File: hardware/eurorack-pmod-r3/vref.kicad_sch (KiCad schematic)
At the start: 6 parts, among them U8 LM4040DBZ-3 VREF, U9 TL072 OP AMP

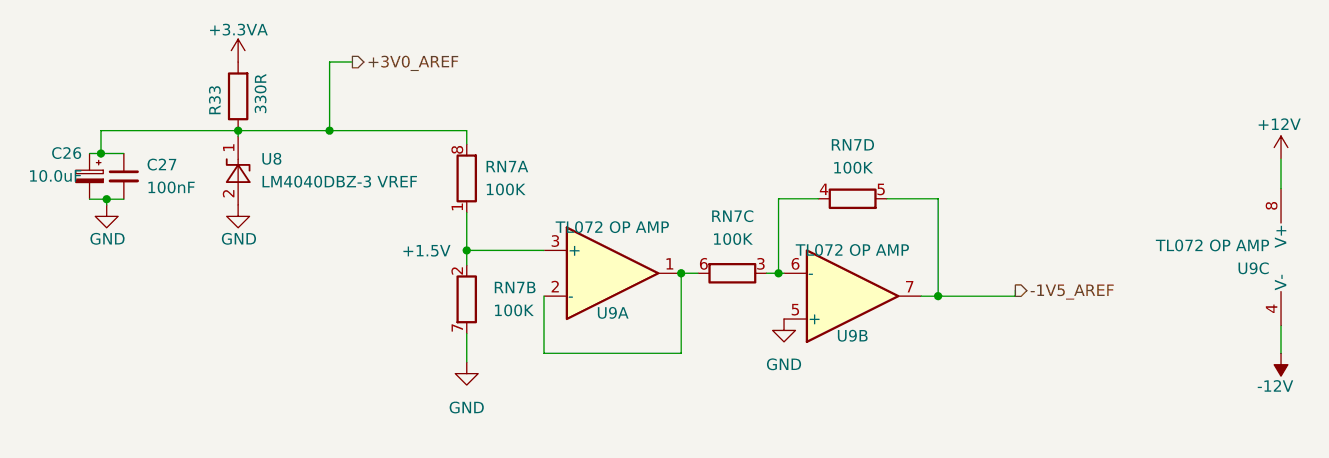
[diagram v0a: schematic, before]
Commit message: try routing with capsense groundfix
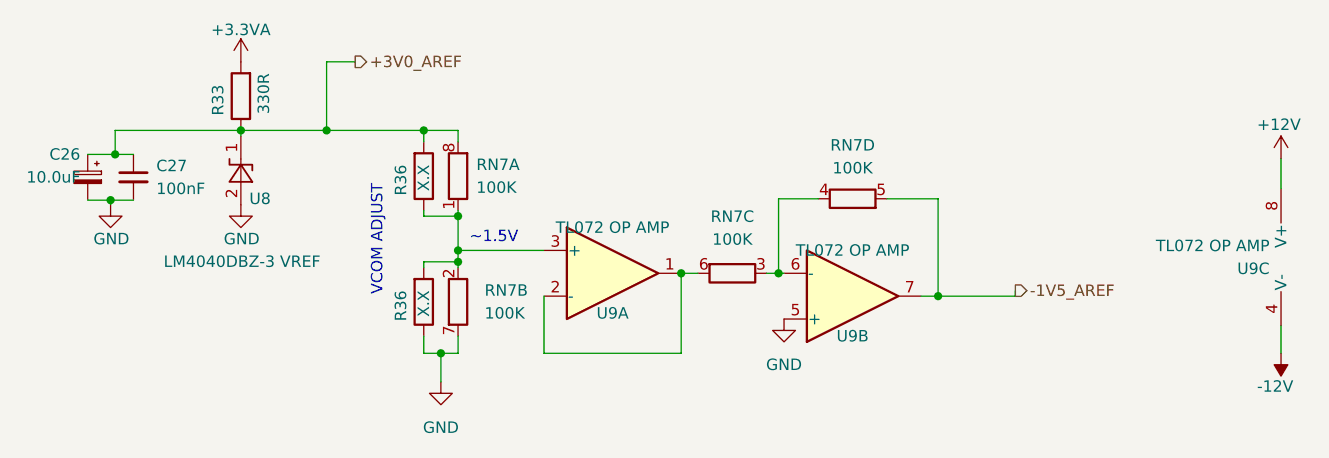
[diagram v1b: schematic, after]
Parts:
- added R36 (x2): X.X, Resistor_SMD:R_0402_1005Metric, symbol Device:R
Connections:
- net +3V0_AREF: now also R36.2
- net GND: now also R36.1
- net at RN7.1 (R1.1), RN7.2 (R2.1): now also R36.1, R36.2; no longer U9.3 (+)
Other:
- note added: "VCOM ADJUST"
- note added: "~1.5V"
- note removed: "+1.5V"
- moved on the sheet: C27, RN7A, RN7B
